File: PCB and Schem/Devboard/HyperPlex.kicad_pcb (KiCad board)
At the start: 2 copper layers, 23.2 x 47.8 mm, 28 parts, among them J1 USB_C_Receptacle_USB2.0_16P, Q1 2N3904, SW1 SW_Push, SW2 SW_SPDT, U1 CH32V203CxTx, U2 TP4056-42-ESOP8, U3 XC6206PxxxMR

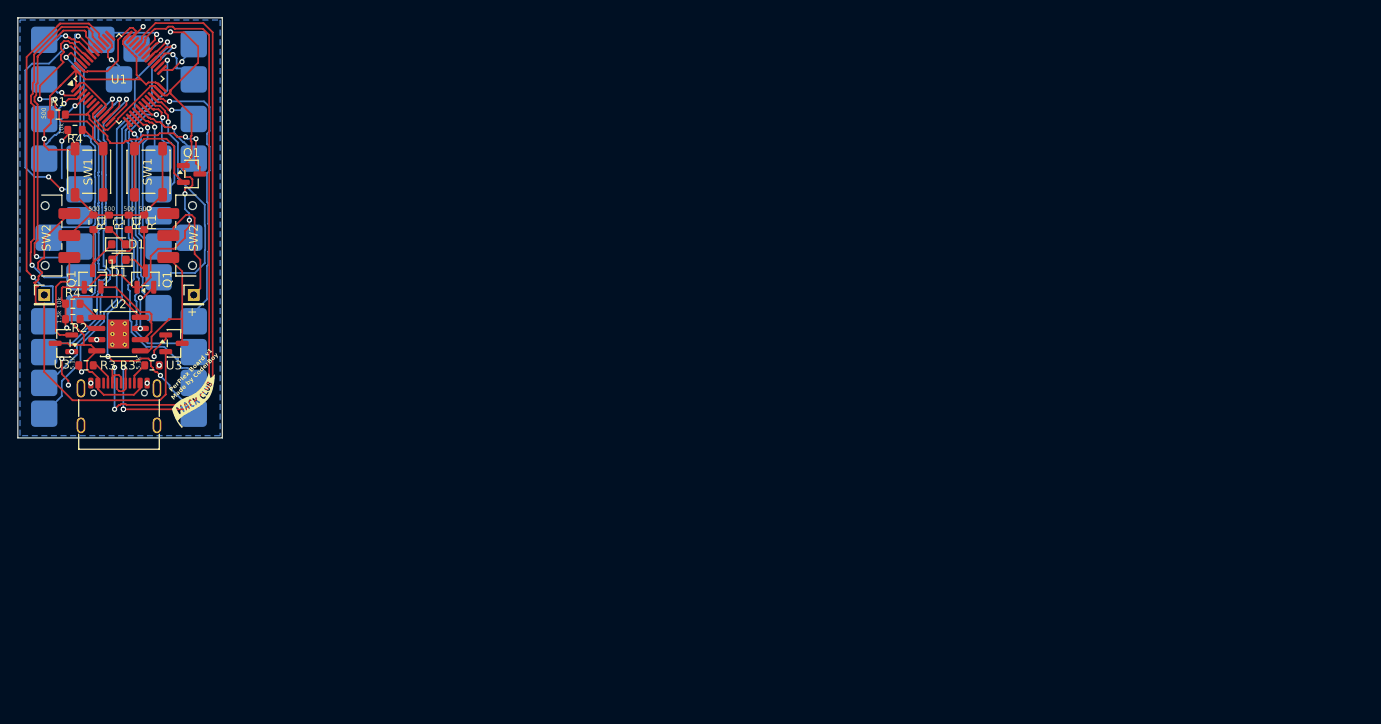
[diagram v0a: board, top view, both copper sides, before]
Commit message: Updated journals, added photos
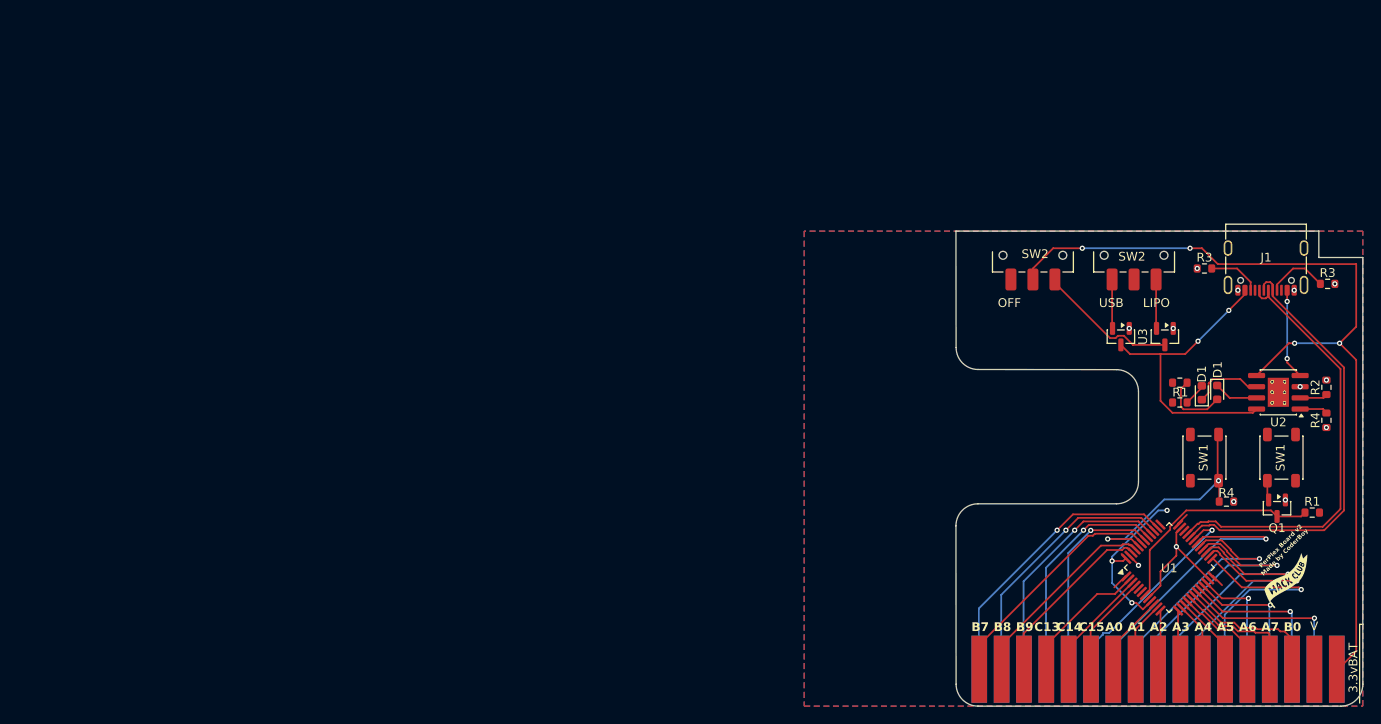
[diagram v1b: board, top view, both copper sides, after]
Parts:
- removed HyperPlex: HyperPlex Connector, HyperPlex:HyperPlex Connector
- removed the Q1 at (39.5, 76.9)
- removed the Q1 at (45.5, 76.9)
- removed the R1 at (39.6, 70.5)
- removed the R1 at (45.4, 70.5)
- removed the REF** at (51.0, 78.8)
- removed the REF** at (34.0, 78.8)
- added REF**: BUS_AT, Connector_PCBEdge:BUS_AT, F.Cu at (180.9, 121.3)
- moved R1 149.6 mm to (178.1, 103.5), turned to 180 degrees
- moved R4 143.1 mm to (179.8, 93.0), turned to -90 degrees
- moved R2 142.7 mm to (179.8, 89.2), turned to 90 degrees
- moved R13 141.4 mm to (179.9, 77.5), turned to 0 degrees
- moved R4 137.5 mm to (168.4, 102.2), turned to 180 degrees
- moved SW1 132.8 mm to (174.6, 97.2)
- moved U2 132.0 mm to (174.3, 89.8), turned to 180 degrees
- moved U1 131.7 mm to (161.9, 109.7)
- moved J1 131.6 mm to (172.9, 74.5), turned to 180 degrees
- moved SW1 130.9 mm to (165.9, 97.2)
- moved Q1 129.1 mm to (174.1, 103.0), turned to -90 degrees
- moved G*** 125.9 mm to (175.4, 111.0)
- moved D1 125.7 mm to (167.3, 89.8), turned to -90 degrees
- moved D1 124.3 mm to (165.6, 89.9), turned to 90 degrees
- moved SW2 123.8 mm to (157.9, 74.2), turned to 180 degrees
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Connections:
- D1 pad 1: Net-(D2-K) -> Net-(Q2-B)
- D1 pad 1: Net-(D1-K) -> Net-(Q1-B)
- U2 pad 5: /3.3VRAW -> +3.3V
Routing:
- net +3.3V: track 13.6 -> 99.4 mm, vias 0 -> 4
- net GND: track 95.4 -> 16.4 mm, vias 15 -> 13
- net /3.3V: track 65.5 -> 24.9 mm, vias 2 -> 3
- net Net-(SW3-A): track 42.0 -> 5.58 mm
- net unconnected-(U1-PA2-Pad12): track 40.4 -> 7.00 mm, vias 1 -> 0
- net unconnected-(U1-PA1-Pad11): track 38.0 -> 8.25 mm, vias 1 -> 0
- net unconnected-(U1-PA9-Pad30): track 5.50 -> 33.5 mm
- net unconnected-(U1-PA15-Pad38): track 5.68 -> 32.5 mm
- net unconnected-(U1-PB15-Pad28): track 54.5 -> 30.7 mm, vias 3 -> 1
- net unconnected-(U1-PB14-Pad27): track 6.91 -> 30.1 mm
- net unconnected-(U1-PB12-Pad25): track 5.71 -> 27.8 mm
- net unconnected-(U1-PA8-Pad29): track 50.4 -> 29.1 mm
- net unconnected-(U1-PB7-Pad43): track 6.46 -> 27.1 mm, vias 1 -> 0
- net /USBDP: track 70.7 -> 50.4 mm, vias 3 -> 0
- net /USBDN: track 70.2 -> 50.1 mm, vias 2 -> 0
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- added copper zone on F.Cu, net /3.3V
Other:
- board size 23.2 x 47.8 mm -> 46.2 x 54 mm
- board text added: "3.3vBAT"
- board text added: "G"
- board text added: "LIPO"
- board text added: "OFF"
- board text added: "PerPlex Board v2 Made by CoderBoy"
- board text added: "USB"
- board text added: "V"
- board text removed: "+"
- board text removed: "1.5k"
- board text removed: "10k"
- board text removed: "3.3V"
- board text removed: "5.1k"
- board text removed: "500"
- board text removed: "GND"
- board text removed: "PerPlex Board v1 Made by CoderBoy"
